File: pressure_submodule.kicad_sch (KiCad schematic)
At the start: 17 parts, among them J3 Conn_01x04, Q1 BSZ0902NSATMA1, U2 INA180

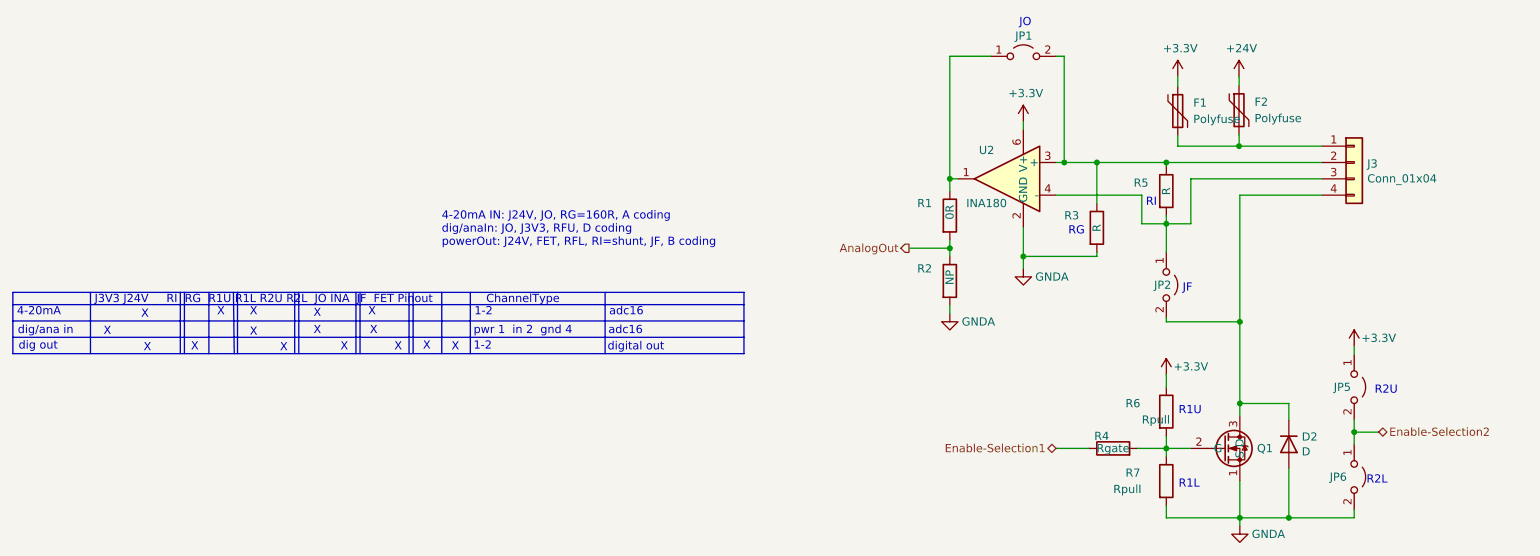
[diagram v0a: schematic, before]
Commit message: WIP
for @Markus
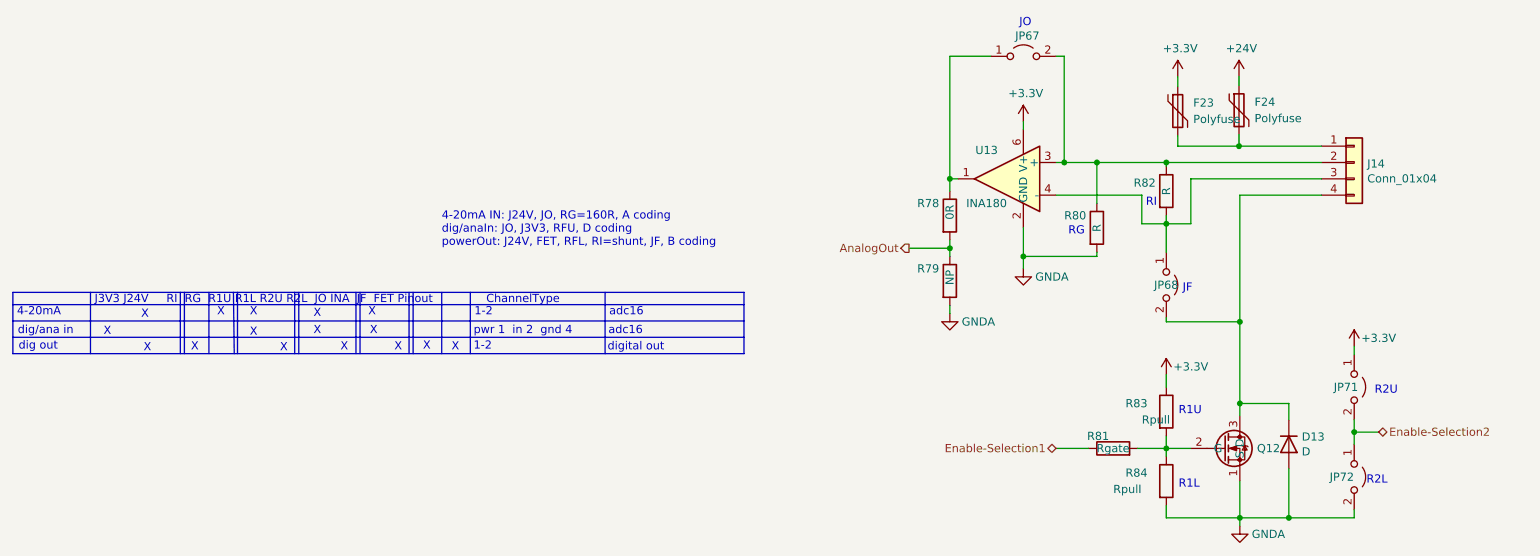
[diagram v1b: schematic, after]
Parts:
- renumbered D2 to D13, F1 to F23, F2 to F24, J3 to J14, JP1 to JP67, JP2 to JP68, JP5 to JP71, JP6 to JP72, Q1 to Q12, R1 to R78, R2 to R79, R3 to R80, R4 to R81, R5 to R82, R6 to R83, R7 to R84, U2 to U13

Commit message: Schematic ready for crosscheck
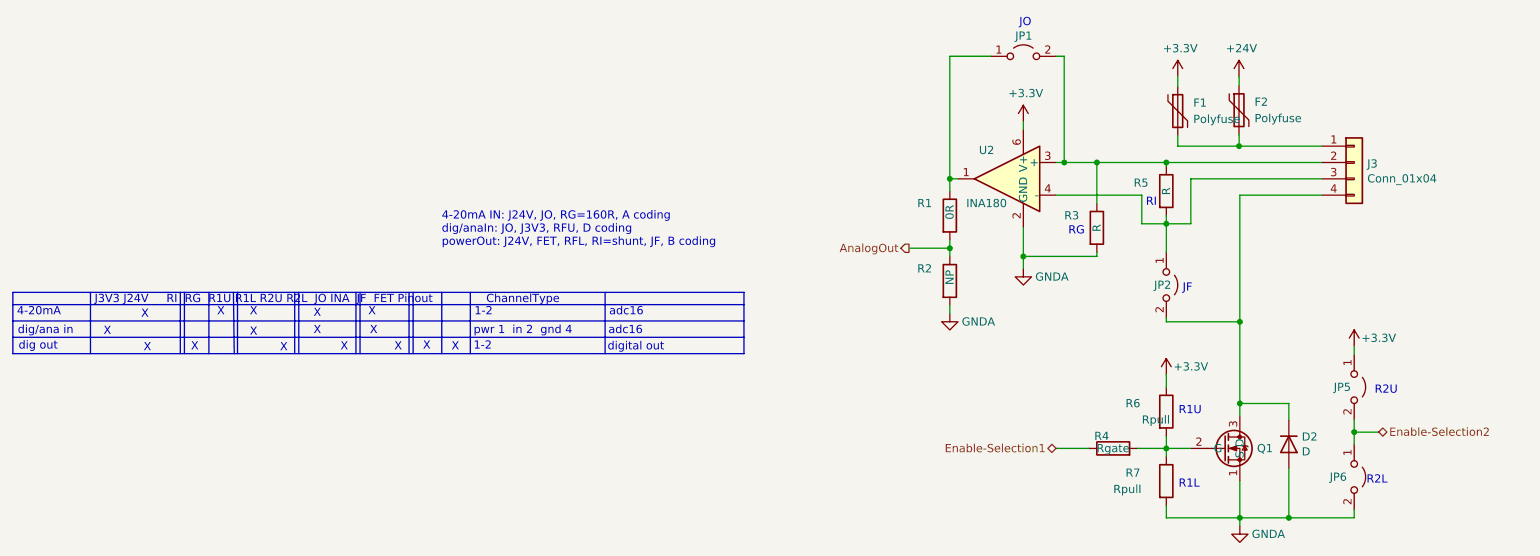
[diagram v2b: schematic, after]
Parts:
- renumbered D13 to D2, F23 to F1, F24 to F2, J14 to J3, JP67 to JP1, JP68 to JP2, JP71 to JP5, JP72 to JP6, Q12 to Q1, R78 to R1, R79 to R2, R80 to R3, R81 to R4, R82 to R5, R83 to R6, R84 to R7, U13 to U2

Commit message: Routing begin
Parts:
- F1, F2: footprint Fuse:Fuse_Littelfuse-LVR125 -> TXV_Library_Footprints:0805L110SL PPTC Polyfuse Littelfuse
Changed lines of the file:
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@@
     (effects (font (size 1.27 1.27)) (justify right))
   )
-  (symbol (lib_id "Connector_Generic:Conn_01x04") (at 241.3 89.281 0) (unit 1)
+  (symbol (lib_id "Connector_Generic:Conn_01x04") (at 241.3 89.281 0)
     (in_bom yes) (on_board yes)
     (property "Reference" "J3" (id 0) (at 243.332 89.4842 0)
@@
     (pin "4")
   )
-  (symbol (lib_id "Jumper:Jumper_2_Open") (at 241.3 124.206 270) (unit 1)
+  (symbol (lib_id "Jumper:Jumper_2_Open") (at 241.3 124.206 270)
     (in_bom yes) (on_board yes)
     (property "Reference" "JP5" (id 0) (at 238.125 124.206 90)
@@
     (pin "2")
   )
-  (symbol (lib_id "Jumper:Jumper_2_Open") (at 241.3 138.176 270) (unit 1)
+  (symbol (lib_id "Jumper:Jumper_2_Open") (at 241.3 138.176 270)
     (in_bom yes) (on_board yes)
     (property "Reference" "JP6" (id 0) (at 237.49 138.176 90)
@@
     (pin "2")
   )
-  (symbol (lib_id "power:+3.3V") (at 213.868 75.946 0) (unit 1)
+  (symbol (lib_id "power:+3.3V") (at 213.868 75.946 0)
     (in_bom yes) (on_board yes)
     (property "Reference" "#PWR017" (id 0) (at 213.868 79.756 0)
@@
     (pin "1")
   )
-  (symbol (lib_id "Device:Polyfuse") (at 223.393 81.153 0) (unit 1)
+  (symbol (lib_id "Device:Polyfuse") (at 223.393 81.153 0)
     (in_bom yes) (on_board yes) (fields_autoplaced)
     (property "Reference" "F2" (id 0) (at 225.806 79.8829 0)
@@
       (effects (font (size 1.27 1.27)) (justify left))
     )
-    (property "Footprint" "Fuse:Fuse_Littelfuse-LVR125" (id 2) (at 224.663 86.233 0)
+    (property "Footprint" "TXV_Library_Footprints:0805L110SL PPTC Polyfuse Littelfuse" (id 2) (at 224.663 86.233 0)
       (effects (font (size 1.27 1.27)) (justify left) hide)
     )
@@
     (pin "2")
   )
-  (symbol (lib_id "Device:R") (at 212.09 138.811 0) (unit 1)
+  (symbol (lib_id "Device:R") (at 212.09 138.811 0)
     (in_bom yes) (on_board yes)
     (property "Reference" "R7" (id 0) (at 205.74 137.541 0)
@@
     (pin "2")
   )
-  (symbol (lib_id "power:+3.3V") (at 241.3 117.856 0) (unit 1)
+  (symbol (lib_id "power:+3.3V") (at 241.3 117.856 0)
     (in_bom yes) (on_board yes)
     (property "Reference" "#PWR020" (id 0) (at 241.3 121.666 0)
@@
     (pin "1")
   )
-  (symbol (lib_id "Device:Polyfuse") (at 213.868 81.28 0) (unit 1)
+  (symbol (lib_id "Device:Polyfuse") (at 213.868 81.28 0)
     (in_bom yes) (on_board yes) (fields_autoplaced)
     (property "Reference" "F1" (id 0) (at 216.281 80.0099 0)
@@
       (effects (font (size 1.27 1.27)) (justify left))
     )
-    (property "Footprint" "Fuse:Fuse_Littelfuse-LVR125" (id 2) (at 215.138 86.36 0)
+    (property "Footprint" "TXV_Library_Footprints:0805L110SL PPTC Polyfuse Littelfuse" (id 2) (at 215.138 86.36 0)
       (effects (font (size 1.27 1.27)) (justify left) hide)
     )
@@
     (pin "2")
   )
-  (symbol (lib_id "power:GNDA") (at 223.52 145.796 0) (unit 1)
+  (symbol (lib_id "power:GNDA") (at 223.52 145.796 0)
     (in_bom yes) (on_board yes)
     (property "Reference" "#PWR019" (id 0) (at 223.52 152.146 0)
@@
     (pin "1")
   )
-  (symbol (lib_id "Jumper:Jumper_2_Open") (at 189.865 72.771 0) (unit 1)
+  (symbol (lib_id "Jumper:Jumper_2_Open") (at 189.865 72.771 0)
     (in_bom yes) (on_board yes)
     (property "Reference" "JP1" (id 0) (at 188.595 69.596 0)
@@
     (pin "2")
   )
-  (symbol (lib_id "power:+24V") (at 223.393 75.946 0) (unit 1)
+  (symbol (lib_id "power:+24V") (at 223.393 75.946 0)
     (in_bom yes) (on_board yes)
     (property "Reference" "#PWR018" (id 0) (at 223.393 79.756 0)
@@
     (pin "1")
   )
-  (symbol (lib_id "Jumper:Jumper_2_Open") (at 212.09 108.331 270) (unit 1)
+  (symbol (lib_id "Jumper:Jumper_2_Open") (at 212.09 108.331 270)
     (in_bom yes) (on_board yes)
     (property "Reference" "JP2" (id 0) (at 210.185 108.331 90)
@@
     (pin "2")
   )
-  (symbol (lib_id "Device:R") (at 178.435 97.536 0) (unit 1)
+  (symbol (lib_id "Device:R") (at 178.435 97.536 0)
     (in_bom yes) (on_board yes)
     (property "Reference" "R1" (id 0) (at 173.355 95.631 0)
@@
     (pin "2")
   )
-  (symbol (lib_id "Device:R") (at 201.295 99.441 0) (unit 1)
+  (symbol (lib_id "Device:R") (at 201.295 99.441 0)
     (in_bom yes) (on_board yes)
     (property "Reference" "R3" (id 0) (at 196.215 97.536 0)
@@
     (pin "2")
   )
-  (symbol (lib_id "Device:R") (at 178.435 107.696 0) (unit 1)
+  (symbol (lib_id "Device:R") (at 178.435 107.696 0)
     (in_bom yes) (on_board yes)
     (property "Reference" "R2" (id 0) (at 173.355 105.791 0)
@@
     (pin "2")
   )
-  (symbol (lib_id "Device:R") (at 212.09 128.016 0) (unit 1)
+  (symbol (lib_id "Device:R") (at 212.09 128.016 0)
     (in_bom yes) (on_board yes)
     (property "Reference" "R6" (id 0) (at 205.74 126.746 0)
@@
     (pin "2")
   )
-  (symbol (lib_id "Device:D") (at 231.14 133.096 270) (unit 1)
+  (symbol (lib_id "Device:D") (at 231.14 133.096 270)
     (in_bom yes) (on_board yes)
     (property "Reference" "D2" (id 0) (at 233.1466 131.9276 90)
@@
     (pin "2")
   )
-  (symbol (lib_id "power:GNDA") (at 178.435 112.776 0) (unit 1)
+  (symbol (lib_id "power:GNDA") (at 178.435 112.776 0)
     (in_bom yes) (on_board yes)
     (property "Reference" "#PWR013" (id 0) (at 178.435 119.126 0)
@@
     (pin "1")
   )
-  (symbol (lib_id "IOB-rescue:INA180-TXV_Library_Symbols") (at 187.325 91.821 0) (mirror y) (unit 1)
+  (symbol (lib_id "IOB-rescue:INA180-TXV_Library_Symbols") (at 187.325 91.821 0) (mirror y)
     (in_bom yes) (on_board yes)
     (property "Reference" "U2" (id 0) (at 184.15 87.376 0))
@@
     (pin "6")
   )
-  (symbol (lib_id "IOB-rescue:BSZ0902NSATMA1-TXV_Library_Symbols") (at 222.25 133.731 0) (unit 1)
+  (symbol (lib_id "IOB-rescue:BSZ0902NSATMA1-TXV_Library_Symbols") (at 222.25 133.731 0)
     (in_bom yes) (on_board yes)
     (property "Reference" "Q1" (id 0) (at 226.187 133.731 0)
@@
     (pin "3")
   )
-  (symbol (lib_id "Device:R") (at 212.09 93.726 0) (unit 1)
+  (symbol (lib_id "Device:R") (at 212.09 93.726 0)
     (in_bom yes) (on_board yes)
     (property "Reference" "R5" (id 0) (at 207.01 92.456 0)
@@
     (pin "2")
   )
-  (symbol (lib_id "power:+3.3V") (at 212.09 122.301 0) (unit 1)
+  (symbol (lib_id "power:+3.3V") (at 212.09 122.301 0)
     (in_bom yes) (on_board yes)
     (property "Reference" "#PWR016" (id 0) (at 212.09 126.111 0)
@@
     (pin "1")
   )
-  (symbol (lib_id "power:GNDA") (at 189.865 105.791 0) (unit 1)
+  (symbol (lib_id "power:GNDA") (at 189.865 105.791 0)
     (in_bom yes) (on_board yes)
     (property "Reference" "#PWR015" (id 0) (at 189.865 112.141 0)
@@
     (pin "1")
   )
-  (symbol (lib_id "Device:R") (at 203.835 133.731 90) (unit 1)
+  (symbol (lib_id "Device:R") (at 203.835 133.731 90)
     (in_bom yes) (on_board yes)
     (property "Reference" "R4" (id 0) (at 203.2 131.826 90)
@@
     (pin "2")
   )
-  (symbol (lib_id "power:+3.3V") (at 189.865 82.931 0) (unit 1)
+  (symbol (lib_id "power:+3.3V") (at 189.865 82.931 0)
     (in_bom yes) (on_board yes)
     (property "Reference" "#PWR014" (id 0) (at 189.865 86.741 0)
